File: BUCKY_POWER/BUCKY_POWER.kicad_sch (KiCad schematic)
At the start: 1 part

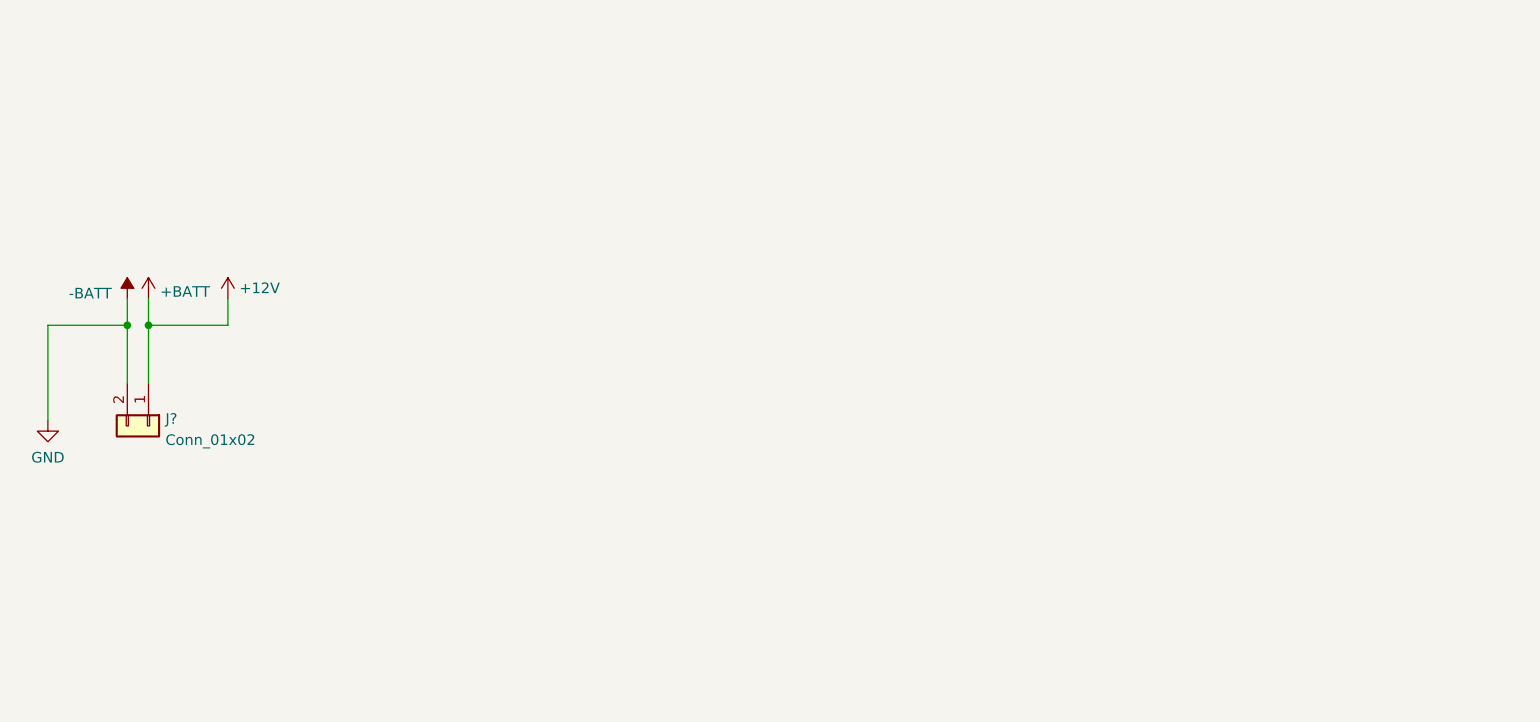
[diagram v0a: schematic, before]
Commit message: Started POWER
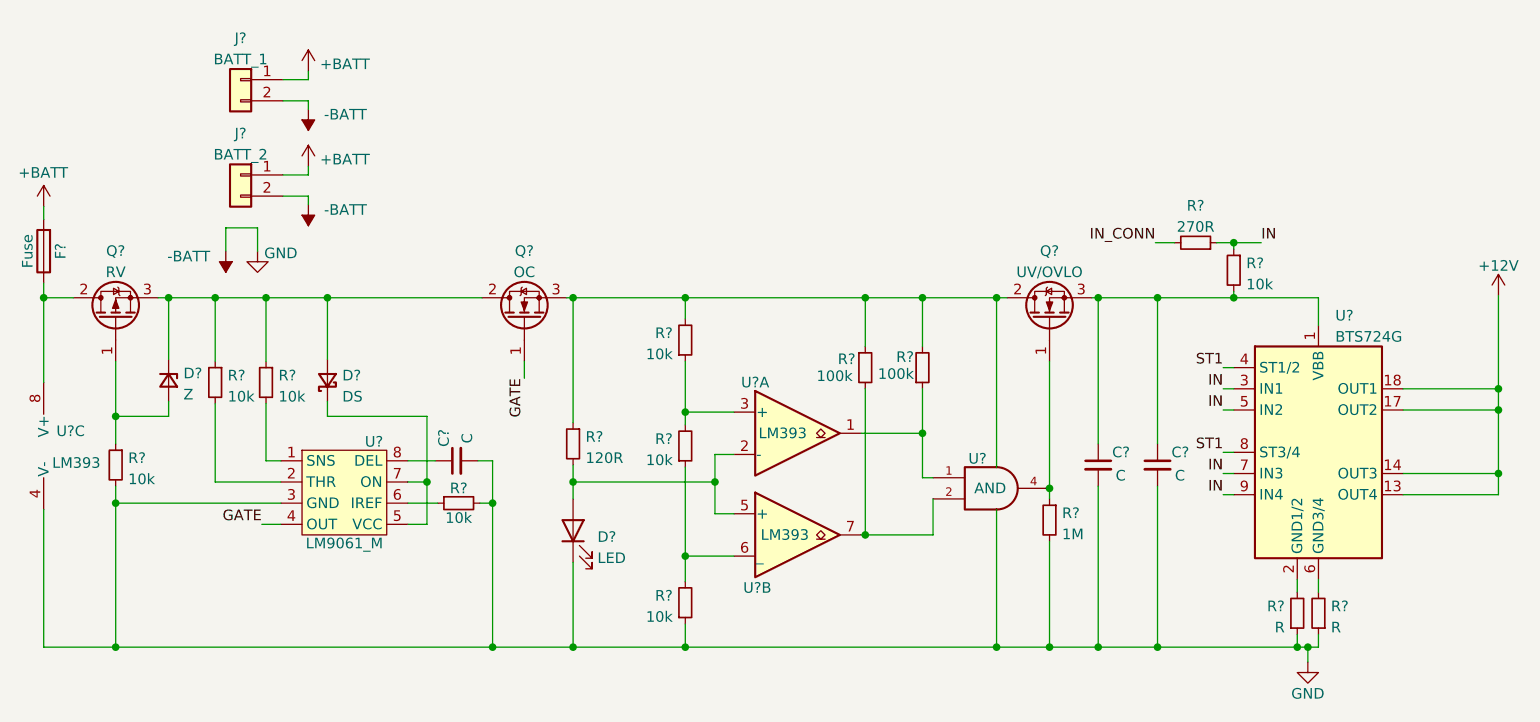
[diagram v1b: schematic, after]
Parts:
- added C? (x3): C, symbol Device:C_Small
- added D?: DS, symbol Device:D_Schottky_Small
- added D?: LED, symbol Device:LED
- added D?: Z, symbol Device:D_Zener_Small
- added F?: Fuse, symbol Device:Fuse
- added J?: BATT_2, symbol Connector_Generic:Conn_01x02
- added Q?: RV, symbol Device:Q_PMOS_GDS
- added Q?: UV/OVLO, symbol Device:Q_NMOS_GDS
- added Q?: OC, symbol Device:Q_NMOS_GDS
- added R? (x8): 10k, symbol Device:R_Small
- added R?: 120R, symbol Device:R_Small
- added R? (x2): 100k, symbol Device:R_Small
- added R? (x2): R, symbol Device:R_Small
- added R?: 270R, symbol Device:R_Small
- added R?: 1M, symbol Device:R_Small
- added U? (x3): LM393, symbol Comparator:LM393
- added U?: LM9061_M, Package_SO:SOIC-8_3.9x4.9mm_P1.27mm, symbol BUCKY_POWER:LM9061_M
- added U?: AND, symbol 74xGxx:74AHC1G08
- added U?: BTS724G, Package_SO:Infineon_PG-DSO-20-32, symbol Power_Management:BTS724G
- J?: value Conn_01x02 -> BATT_1
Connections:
- net +12V: now also U?.13 (OUT4), U?.14 (OUT3), U?.17 (OUT2), U?.18 (OUT1); no longer J?.1 (Pin_1)
- net -BATT: now also C?.2, C?.2, C?.2, D?.1 (K), J?.2 (Pin_2), R?.1, R?.1, R?.1, R?.2, R?.2, R?.2, U?.3 (GND), U?.3 (GND), U?.4 (V-)
- new net: R?.1, R?.2, U?.6 (_)
- new net: R?.1, R?.2, U?.3 (+)
- new net: D?.2 (A), R?.2, U?.2 (-), U?.5 (+)
- new net: R?.2, U?.2, U?.7
- new net: C?.1, U?.8 (DEL)
- new net: D?.1 (K), U?.5 (VCC), U?.7 (ON)
- new net: D?.1 (K), D?.2 (A), Q?.2 (D), Q?.3 (S), R?.1, R?.1
- new net: R?.2, U?.2 (THR)
- new net: D?.2 (A), Q?.1 (G), R?.1
- new net: F?.1, Q?.2 (D), U?.8 (V+)
- new net: R?.2, U?.2 (GND1/2)
- new net: R?.2, U?.1 (SNS)
- new net: R?.1, U?.6 (IREF)
- new net: R?.1, U?.1, U?.1
- new net: Q?.1 (G), R?.1, U?.4
- new net: C?.1, C?.1, Q?.3 (S), R?.2, U?.1 (VBB), U?.10 (VBB), U?.11 (VBB), U?.12 (VBB), U?.15 (VBB), U?.16 (VBB), U?.19 (VBB), U?.20 (VBB)
- new net: R?.2, U?.6 (GND3/4)
- new net +BATT: F?.2, J?.1 (Pin_1), J?.1 (Pin_1)
- new net GATE: Q?.1 (G), U?.4 (OUT)
- new net IN: R?.1, R?.1, U?.3 (IN1), U?.5 (IN2), U?.7 (IN3), U?.9 (IN4)
- new net IN_CONN: R?.2
- new net ST1: U?.4 (ST1/2), U?.8 (ST3/4)
- new net VCC: Q?.2 (D), Q?.3 (S), R?.1, R?.1, R?.2, R?.2, U?.5 (VCC)
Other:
- moved on the sheet: J?

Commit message: Power Done
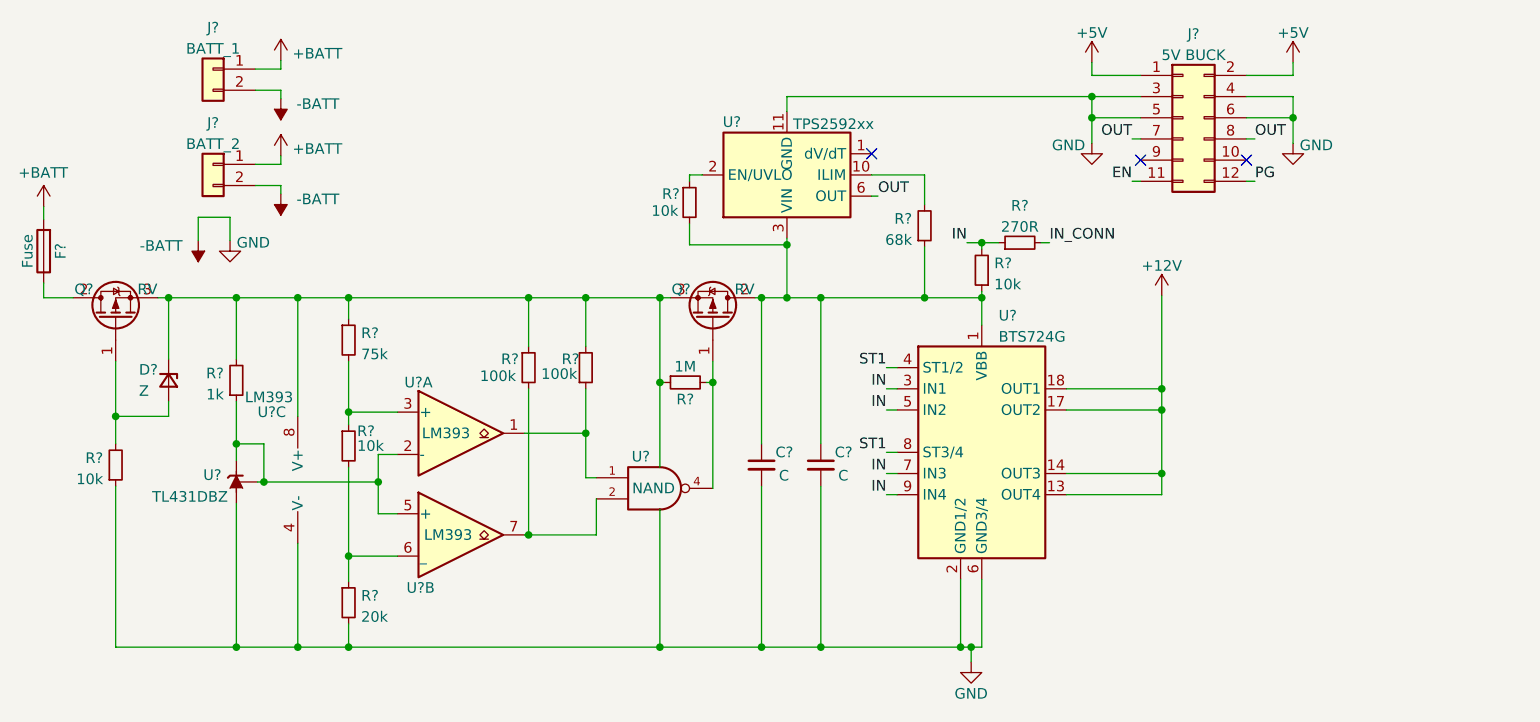
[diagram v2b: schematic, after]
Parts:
- removed C?: C, symbol Device:C_Small
- removed D?: DS, symbol Device:D_Schottky_Small
- removed D?: LED, symbol Device:LED
- removed Q?: UV/OVLO, symbol Device:Q_NMOS_GDS
- removed Q?: OC, symbol Device:Q_NMOS_GDS
- removed R?: 120R, symbol Device:R_Small
- removed R? (x3): 10k, symbol Device:R_Small
- removed R? (x2): R, symbol Device:R_Small
- removed U?: LM9061_M, Package_SO:SOIC-8_3.9x4.9mm_P1.27mm, symbol BUCKY_POWER:LM9061_M
- removed U?: AND, symbol 74xGxx:74AHC1G08
- added J?: 5V BUCK, symbol Connector_Generic:Conn_02x06_Odd_Even
- added Q?: RV, symbol Device:Q_PMOS_GDS
- added R?: 68k, symbol Device:R_Small
- added R?: 1k, symbol Device:R_Small
- added R?: 10k, symbol Device:R_Small
- added U?: NAND, symbol 74xGxx:74AHC1G00
- added U?: TL431DBZ, Package_TO_SOT_SMD:SOT-23, symbol Reference_Voltage:TL431DBZ
- added U?: TPS2592xx, Package_SON:VSON-10-1EP_3x3mm_P0.5mm_EP1.65x2.4mm_ThermalVias, symbol Power_Management:TPS2592xx
- R?: value 10k -> 20k
- R?: value 10k -> 75k
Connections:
- net -BATT: now also R?.1, R?.2, U?.2 (GND1/2), U?.6 (GND3/4), J?.3 (Pin_3), J?.4 (Pin_4), J?.5 (Pin_5), J?.6 (Pin_6), U?.11 (GND), U?.3 (A), U?.3 (GND); no longer R?.1, R?.2, R?.2
- net IN: now also R?.2; no longer R?.1
- net VCC: now also D?.1 (K), Q?.3 (S), R?.1, R?.1, U?.8 (V+), Q?.3 (S), R?.2, U?.5 (VCC); no longer R?.2
- net at U?.2 (-), U?.5 (+): now also R?.1, U?.1 (K), U?.2 (REF)
- net at R?.2, U?.7: now also U?.2
- net at D?.2 (A), Q?.1 (G): now also R?.2; no longer R?.1
- net at F?.1, Q?.2 (D): no longer U?.8 (V+)
- net at R?.1, U?.1: now also U?.1
- net at C?.1, C?.1, U?.1 (VBB)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: now also R?.1, Q?.2 (D), R?.1, R?.2, U?.3 (VIN), U?.4 (VIN), U?.5 (VIN); no longer R?.2
- new net: R?.1, R?.2, U?.6 (_)
- new net: R?.1, R?.2, U?.3 (+)
- new net: R?.2, U?.10 (ILIM)
- new net: Q?.1 (G), R?.2, U?.4
- new net: R?.1, U?.2 (EN/UVLO)
- new net +5V: J?.1 (Pin_1), J?.2 (Pin_2)
- new net EN: J?.11 (Pin_11)
- new net OUT: J?.7 (Pin_7), J?.8 (Pin_8), U?.6 (OUT), U?.7 (OUT), U?.8 (OUT)
- new net PG: J?.12 (Pin_12)
- no-connect marks 0 -> 3
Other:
- moved on the sheet: C?, J?, R?, U?, U?A, U?B, U?C
